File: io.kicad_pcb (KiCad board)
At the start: 2 copper layers, 182 x 129 mm, 37 parts, among them CON1 AVR_ISP, IC1 ATMEGA644P-P, J1 DB9, J2 DB9, P1 CONN_CTL_DATA, P2 CONN_ADDR, P3 SLOT1, P4 SLOT2, P5 SLOT3, P6 SLOT4, P7 SLOT_EX_ADDR, U1 74LS138, U2 74HC245, U3 DISP_5110, U5 74HC05, U6 MAX232, Y1 14.7456M

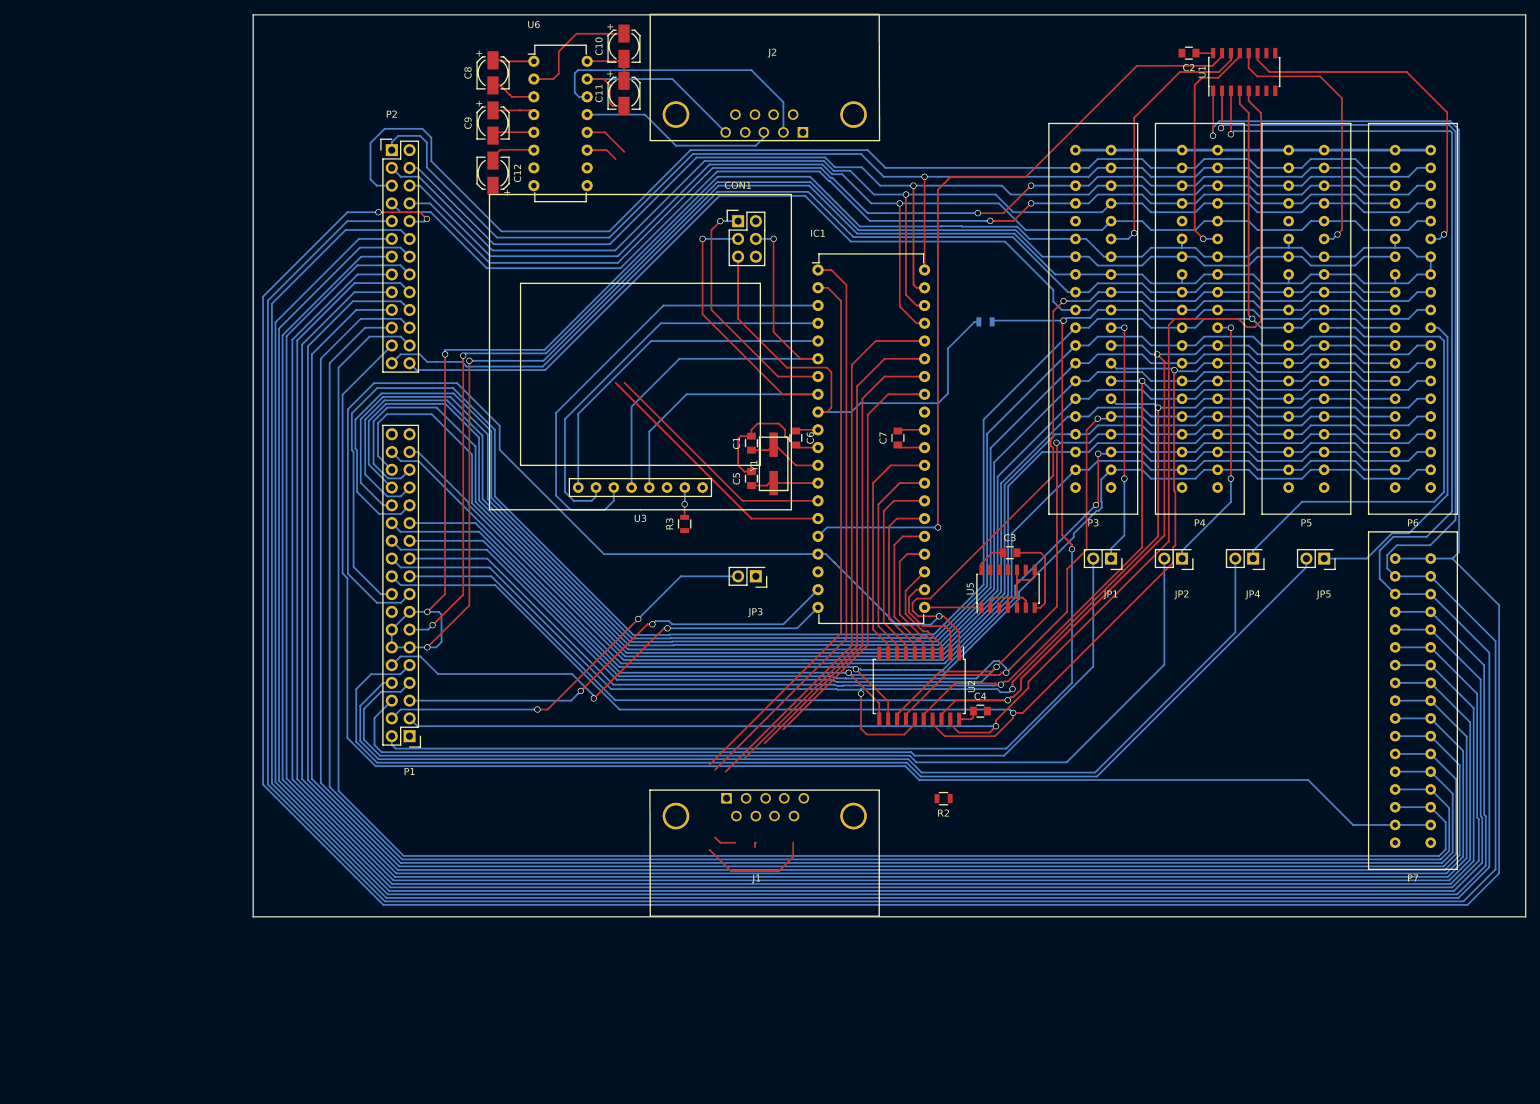
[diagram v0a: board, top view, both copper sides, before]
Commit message: new layout
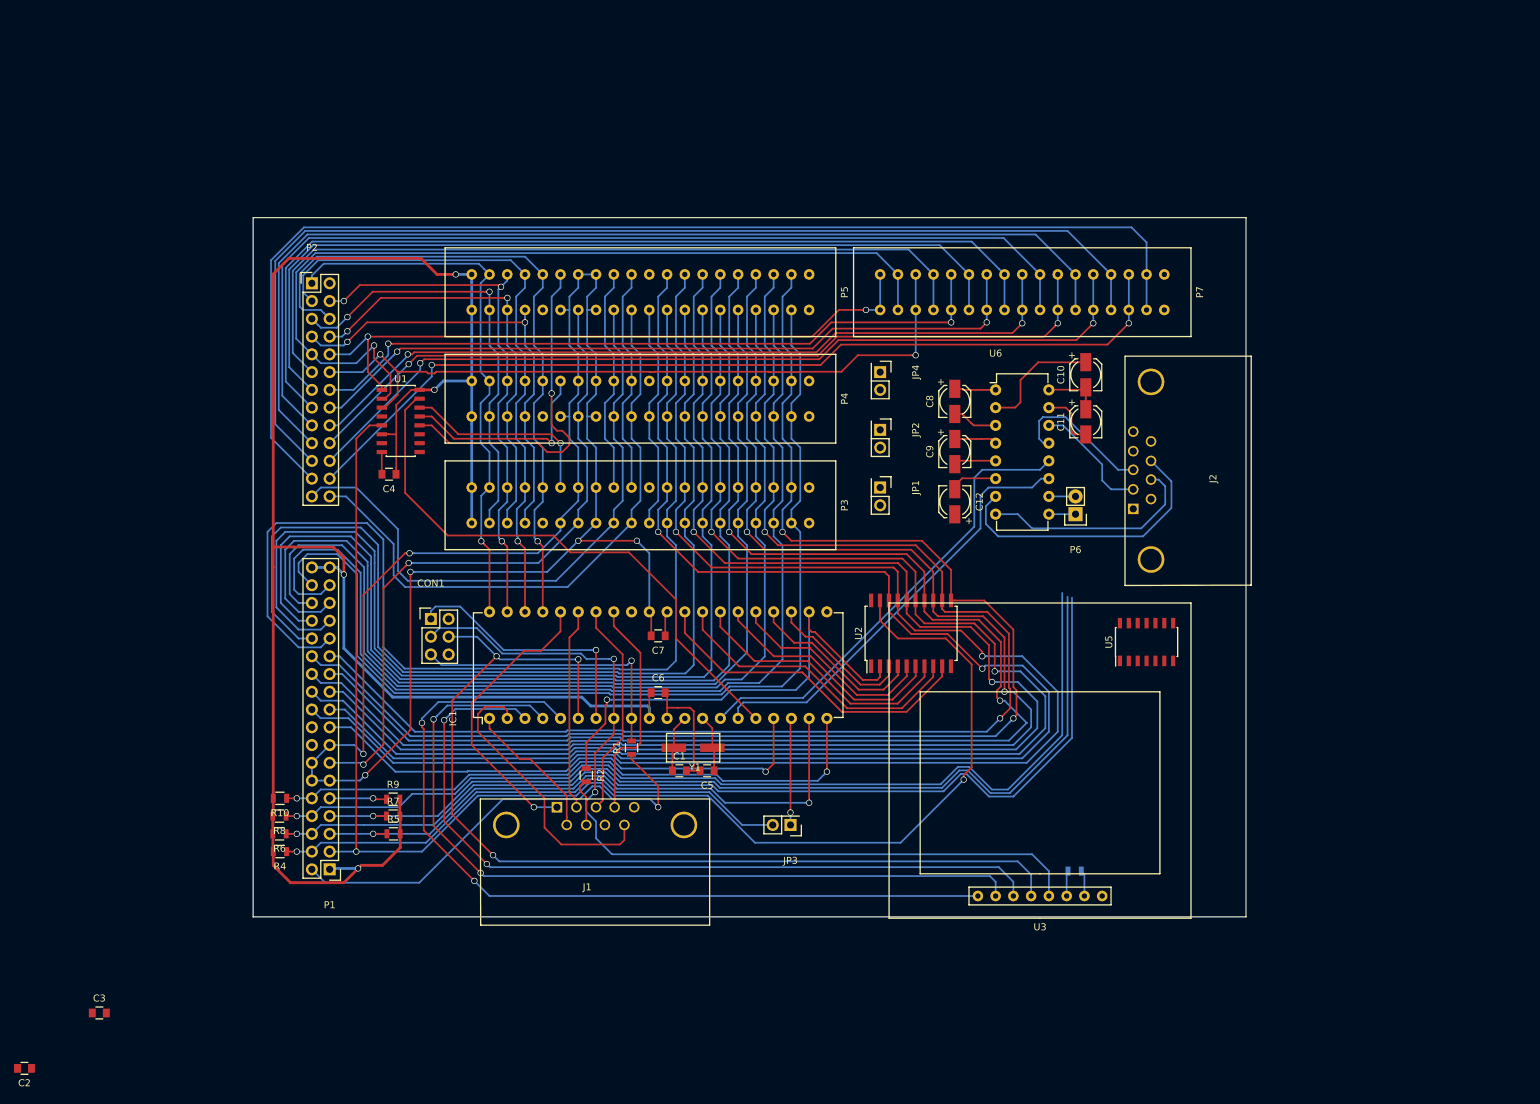
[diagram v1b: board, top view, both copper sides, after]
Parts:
- removed JP5: INT_S4, Pin_Headers:Pin_Header_Straight_2x01
- added R10: 4.7k, Resistors_SMD:R_0805, F.Cu at (20.8, 146.1)
- added R4: 4.7k, Resistors_SMD:R_0805, F.Cu at (20.8, 153.7)
- added R5: 4.7k, Resistors_SMD:R_0805, F.Cu at (37.1, 151.1)
- added R6: 4.7k, Resistors_SMD:R_0805, F.Cu at (20.8, 151.1)
- added R7: 4.7k, Resistors_SMD:R_0805, F.Cu at (37.0, 148.6)
- added R8: 4.7k, Resistors_SMD:R_0805, F.Cu at (20.8, 148.6)
- added R9: 4.7k, Resistors_SMD:R_0805, F.Cu at (37.0, 146.2)
- P6: value SLOT4 -> CONN_01X02; footprint m68kcomp1:edgecon_2x20 -> Pin_Headers:Pin_Header_Straight_1x02
- R1: moved to F.Cu
- R3: moved to B.Cu
- moved C2 221.0 mm to (-15.7, 184.7)
- moved C3 145.9 mm to (-5.00, 176.8)
- moved U1 130.6 mm to (38.1, 92.1), turned to 0 degrees
- moved P5 95.3 mm to (72.4, 73.7), turned to 90 degrees
- moved C4 91.1 mm to (36.4, 99.7), turned to 180 degrees
- moved U3 81.7 mm to (129.5, 160.0)
- moved C10 81.1 mm to (136.1, 85.5)
- moved C11 81.1 mm to (136.1, 92.2)
- moved C12 81.1 mm to (117.3, 103.6)
- moved C8 81.1 mm to (117.3, 89.3)
- moved C9 81.1 mm to (117.3, 96.5)
- moved U6 81.1 mm to (123.2, 87.6)
- moved P7 80.8 mm to (127.0, 73.7), turned to 90 degrees
- moved P4 80.8 mm to (72.4, 88.9), turned to 90 degrees
- moved IC1 79.5 mm to (50.8, 134.6), turned to 90 degrees
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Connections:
- net Net-(J2-Pad2) renamed /RS232_TX
- net Net-(J2-Pad3) renamed /RS232_RX
- J2 pad 7: (no net) -> /RS232_RTS
- J2 pad 8: (no net) -> /RS232_CTS
- P6 pad 1: VCC -> /RTS
- P6 pad 2: VCC -> /CTS
- U1 pad 11: /~EN_S4 -> (no net)
- U5 pad 10: /~DTACK -> (no net)
- U5 pad 11: Net-(P6-Pad9) -> GND
- U6 pad 10: (no net) -> /CTS
- U6 pad 7: (no net) -> /RS232_CTS
- U6 pad 8: (no net) -> /RS232_RTS
- U6 pad 9: (no net) -> /RTS
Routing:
- net /A8: track 448.4 -> 94.9 mm, vias 3 -> 2
- net /A10: track 435.6 -> 105.1 mm, vias 1 -> 2
- net /A9: track 437.3 -> 126.0 mm
- net /~AS: track 268.6 -> 32.6 mm, vias 1 -> 0
- net VCC: track 76.7 -> 303.9 mm, vias 0 -> 4
- net GND: track 499.2 -> 273.1 mm, vias 4 -> 6
- net /A12: track 310.4 -> 100.7 mm, vias 0 -> 2
- net /A11: track 313.4 -> 115.1 mm
- net /A14: track 298.6 -> 105.9 mm, vias 0 -> 2
- net /A13: track 301.3 -> 124.0 mm
- net /A16: track 286.6 -> 112.2 mm, vias 0 -> 2
- net /~IRQ6: track 168.2 -> 8.18 mm, vias 0 -> 1
- net /A15: track 289.3 -> 132.9 mm
- net /A18: track 274.5 -> 118.2 mm, vias 0 -> 2
- net /~WR: track 259.4 -> 107.2 mm, vias 2 -> 1
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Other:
- board size 182 x 129 mm -> 142 x 100 mm
